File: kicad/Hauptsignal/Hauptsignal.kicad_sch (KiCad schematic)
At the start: 17 parts, among them J0 VCC, J1 VkzBw, J2 ROT, J4 GRÜN, J5 Zs7-3, J6 Ra, J7 Zs7-1, J8 Zs7-2, J9 Ra/Zs1

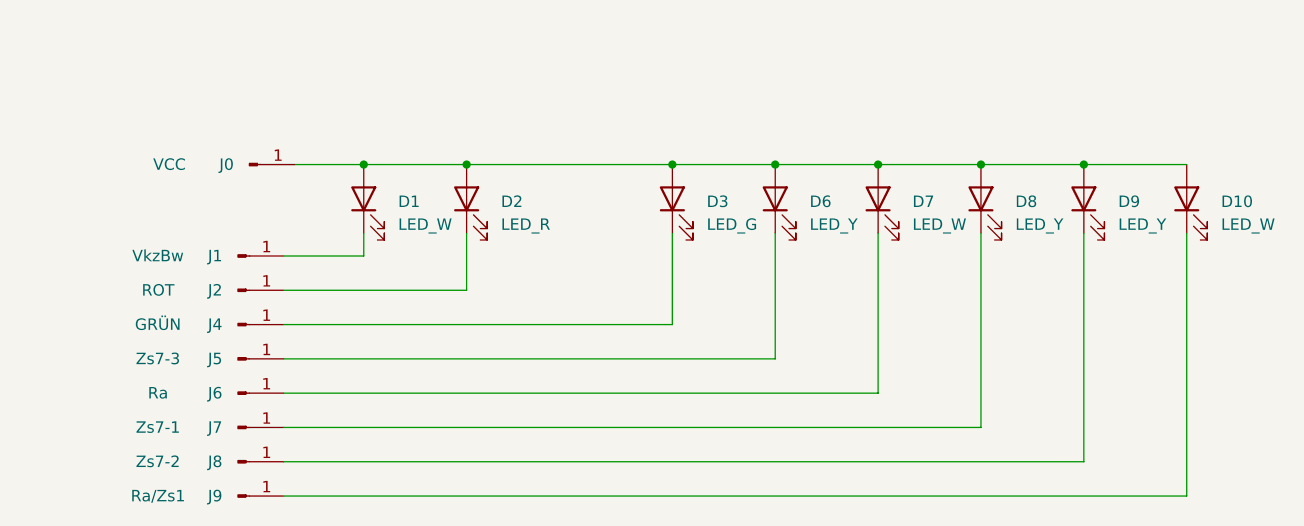
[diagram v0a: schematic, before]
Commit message: Add CC-BY-SA 4.0 license
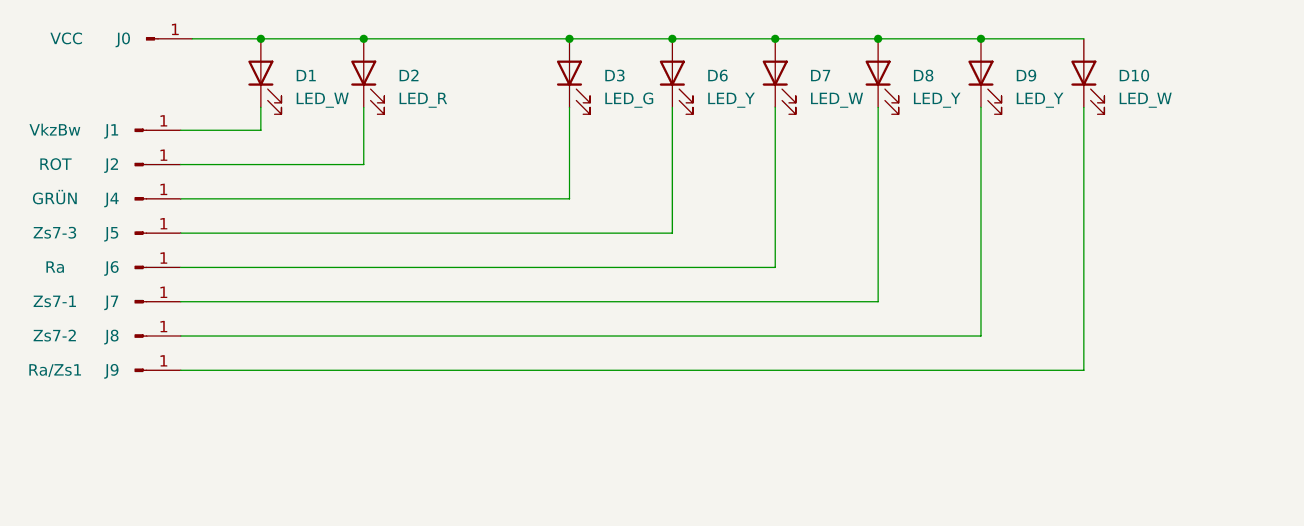
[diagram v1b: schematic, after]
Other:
- title: (none) -> KS-Hauptsignal
- moved on the sheet: D1, D10, D2, D3, D6, D7, D8, D9, J0, J1, J2, J4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
